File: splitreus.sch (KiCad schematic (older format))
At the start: 101 parts, among them J1 TRRS, J2 battery, SW0 SW_PUSH, SW1 SW_PUSH, SW10 SW_PUSH, SW11 SW_PUSH, SW12 SW_PUSH, SW13 SW_PUSH, SW14 SW_PUSH, SW15 SW_PUSH, SW16 SW_PUSH, SW17 SW_PUSH, SW18 SW_PUSH, SW19 SW_PUSH, SW2 SW_PUSH, SW20 SW_PUSH, SW21 SW_PUSH, SW22 SW_PUSH, SW23 SW_PUSH, SW24 SW_PUSH, SW25 SW_PUSH, SW26 SW_PUSH, SW27 SW_PUSH, SW28 SW_PUSH, SW29 SW_PUSH, SW3 SW_PUSH, SW30 SW_PUSH, SW4 SW_PUSH, SW5 SW_PUSH, SW6 SW_PUSH, SW7 SW_PUSH, SW8 SW_PUSH, SW9 SW_PUSH, U0 ProMicro, U1 HOLE, U2 HOLE, U3 HOLE, U4 HOLE

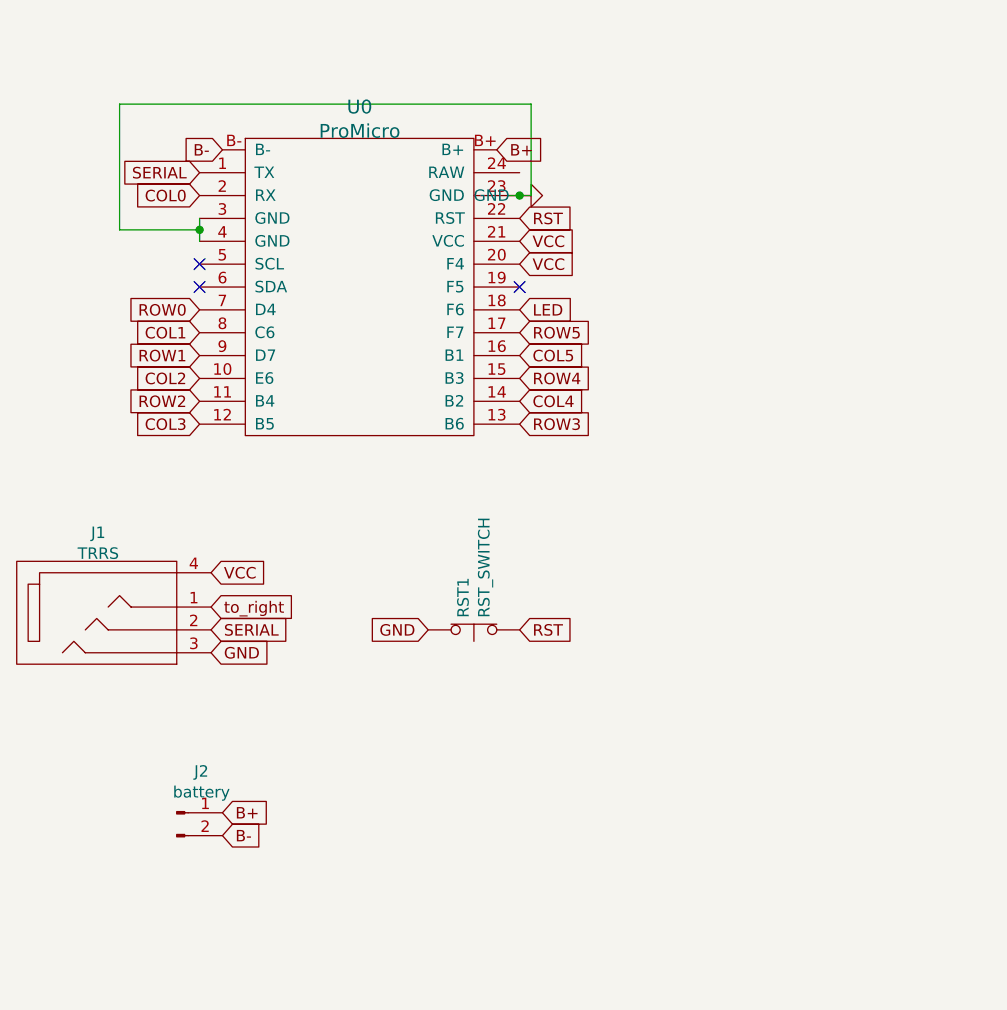
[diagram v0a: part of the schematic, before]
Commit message: fin?
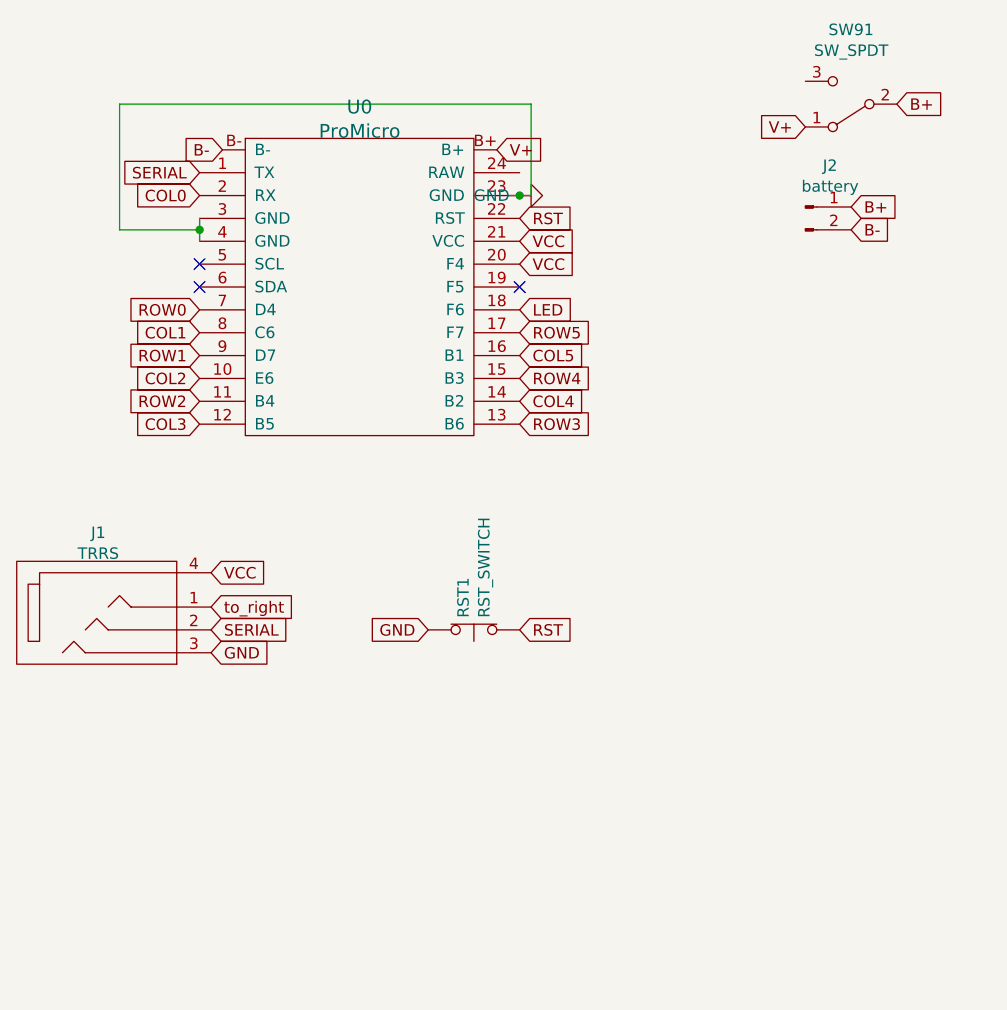
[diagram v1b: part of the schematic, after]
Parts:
- added SW91: SW_SPDT, Custom Footies:reversible_power, symbol Switch:SW_SPDT
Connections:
- net B+: now also SW91.2 (B); no longer U0.B+
- new net V+: SW91.1 (A), U0.B+
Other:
- moved on the sheet: J2
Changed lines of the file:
@@
 Text GLabel 9200 1500 0    50   Input ~ 0
 SERIAL
-Text GLabel 10500 1400 2    50   Input ~ 0
-B+
 Text GLabel 9300 1400 0    50   Input ~ 0
 B-
@@
 L Connector:Conn_01x02_Male J2
 U 1 1 60595BC7
-P 9100 4300
-F 0 "J2" H 9208 4481 50  0000 C CNN
-F 1 "battery" H 9208 4390 50  0000 C CNN
-F 2 "Connector_PinSocket_2.54mm:PinSocket_1x02_P2.54mm_Vertical" H 9100 4300 50  0001 C CNN
-F 3 "~" H 9100 4300 50  0001 C CNN
-	1    9100 4300
+P 11850 1650
+F 0 "J2" H 11958 1831 50  0000 C CNN
+F 1 "battery" H 11958 1740 50  0000 C CNN
+F 2 "Connector_PinSocket_2.54mm:PinSocket_1x02_P2.54mm_Vertical" H 11850 1650 50  0001 C CNN
+F 3 "~" H 11850 1650 50  0001 C CNN
+	1    11850 1650
 	1    0    0    -1
 $EndComp
-Text GLabel 9300 4300 2    50   Input ~ 0
-B+
-Text GLabel 9300 4400 2    50   Input ~ 0
+Text GLabel 12050 1750 2    50   Input ~ 0
 B-
 $Comp
@@
 	1    0    0    -1
 $EndComp
+Text GLabel 12250 1200 2    50   Input ~ 0
+B+
+$Comp
+L Switch:SW_SPDT SW91
+U 1 1 60684D01
+P 12050 1200
+F 0 "SW91" H 12050 875 50  0000 C CNN
+F 1 "SW_SPDT" H 12050 966 50  0000 C CNN
+F 2 "Custom Footies:reversible_power" H 12050 1200 50  0001 C CNN
+F 3 "~" H 12050 1200 50  0001 C CNN
+	1    12050 1200
+	-1   0    0    1
+$EndComp
+Text GLabel 12050 1650 2    50   Input ~ 0
+B+
+Text GLabel 11850 1300 0    50   Input ~ 0
+V+
+Text GLabel 10500 1400 2    50   Input ~ 0
+V+
 $EndSCHEMATC

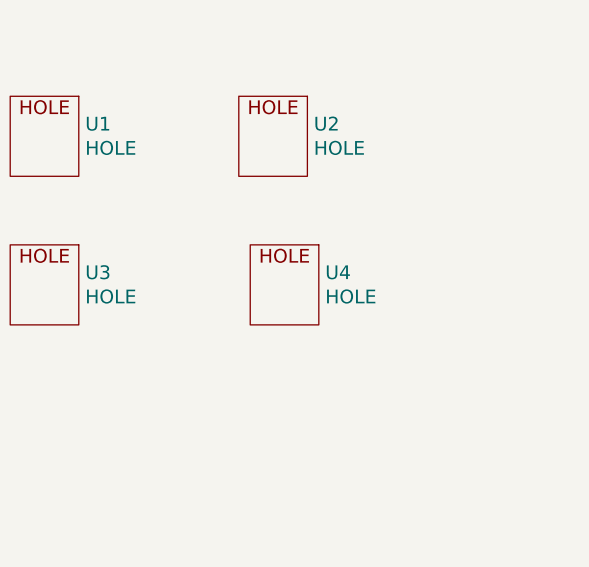
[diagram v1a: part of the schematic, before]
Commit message: moved stuff
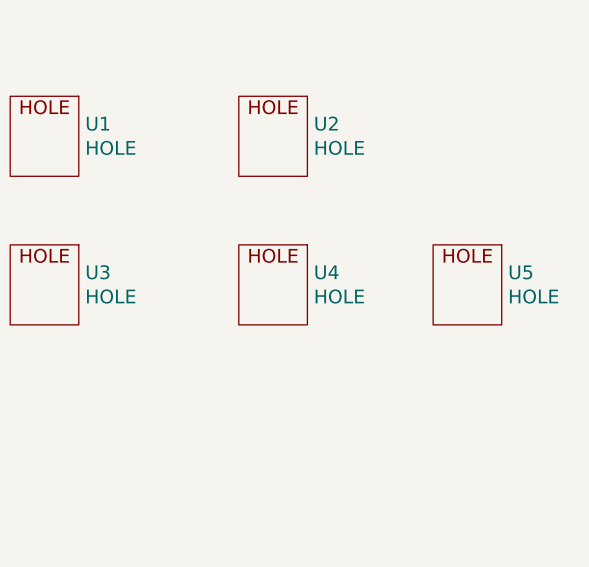
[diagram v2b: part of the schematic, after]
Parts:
- added U5: HOLE, MountingHole:MountingHole_2.2mm_M2_DIN965, symbol hole:HOLE
- U1, U2, U3, U4: footprint MountingHole:MountingHole_2.2mm_M2_DIN965_Pad -> MountingHole:MountingHole_2.2mm_M2_DIN965
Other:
- moved on the sheet: U4
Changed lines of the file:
@@
 F 0 "U1" H 11328 6628 60  0000 L CNN
 F 1 "HOLE" H 11328 6522 60  0000 L CNN
-F 2 "MountingHole:MountingHole_2.2mm_M2_DIN965_Pad" H 11150 6550 60  0001 C CNN
+F 2 "MountingHole:MountingHole_2.2mm_M2_DIN965" H 11150 6550 60  0001 C CNN
 F 3 "" H 11150 6550 60  0000 C CNN
 	1    11150 6550
@@
 F 0 "U2" H 12328 6628 60  0000 L CNN
 F 1 "HOLE" H 12328 6522 60  0000 L CNN
-F 2 "MountingHole:MountingHole_2.2mm_M2_DIN965_Pad" H 12150 6550 60  0001 C CNN
+F 2 "MountingHole:MountingHole_2.2mm_M2_DIN965" H 12150 6550 60  0001 C CNN
 F 3 "" H 12150 6550 60  0000 C CNN
 	1    12150 6550
@@
 F 0 "U3" H 11328 7278 60  0000 L CNN
 F 1 "HOLE" H 11328 7172 60  0000 L CNN
-F 2 "MountingHole:MountingHole_2.2mm_M2_DIN965_Pad" H 11150 7200 60  0001 C CNN
+F 2 "MountingHole:MountingHole_2.2mm_M2_DIN965" H 11150 7200 60  0001 C CNN
 F 3 "" H 11150 7200 60  0000 C CNN
 	1    11150 7200
@@
 L hole:HOLE U4
 U 1 1 6066B2B8
-P 12200 7200
-F 0 "U4" H 12378 7278 60  0000 L CNN
-F 1 "HOLE" H 12378 7172 60  0000 L CNN
-F 2 "MountingHole:MountingHole_2.2mm_M2_DIN965_Pad" H 12200 7200 60  0001 C CNN
-F 3 "" H 12200 7200 60  0000 C CNN
-	1    12200 7200
+P 12150 7200
+F 0 "U4" H 12328 7278 60  0000 L CNN
+F 1 "HOLE" H 12328 7172 60  0000 L CNN
+F 2 "MountingHole:MountingHole_2.2mm_M2_DIN965" H 12150 7200 60  0001 C CNN
+F 3 "" H 12150 7200 60  0000 C CNN
+	1    12150 7200
 	1    0    0    -1
 $EndComp
@@
 Text GLabel 10500 1400 2    50   Input ~ 0
 V+
+$Comp
+L hole:HOLE U5
+U 1 1 614B0606
+P 13000 7200
+F 0 "U5" H 13178 7278 60  0000 L CNN
+F 1 "HOLE" H 13178 7172 60  0000 L CNN
+F 2 "MountingHole:MountingHole_2.2mm_M2_DIN965" H 13000 7200 60  0001 C CNN
+F 3 "" H 13000 7200 60  0000 C CNN
+	1    13000 7200
+	1    0    0    -1
+$EndComp
 $EndSCHEMATC
